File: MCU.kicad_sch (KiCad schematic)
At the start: 10 parts

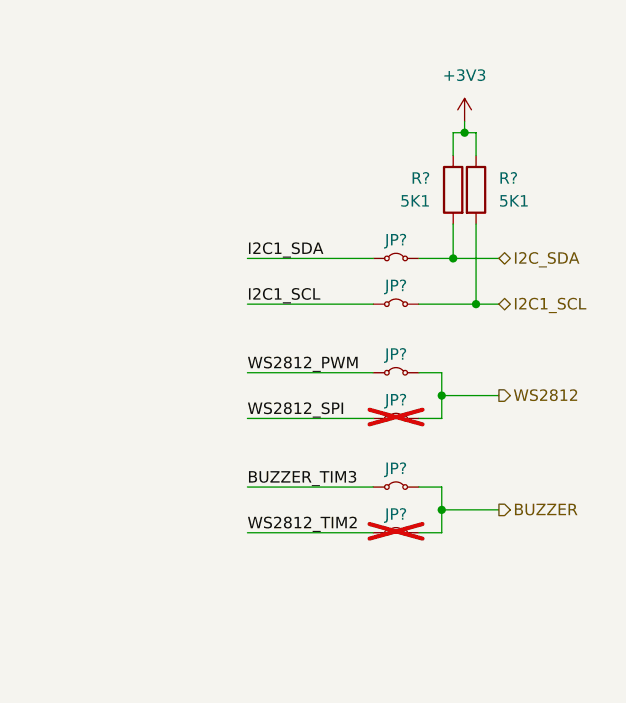
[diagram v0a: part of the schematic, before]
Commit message: Small changes
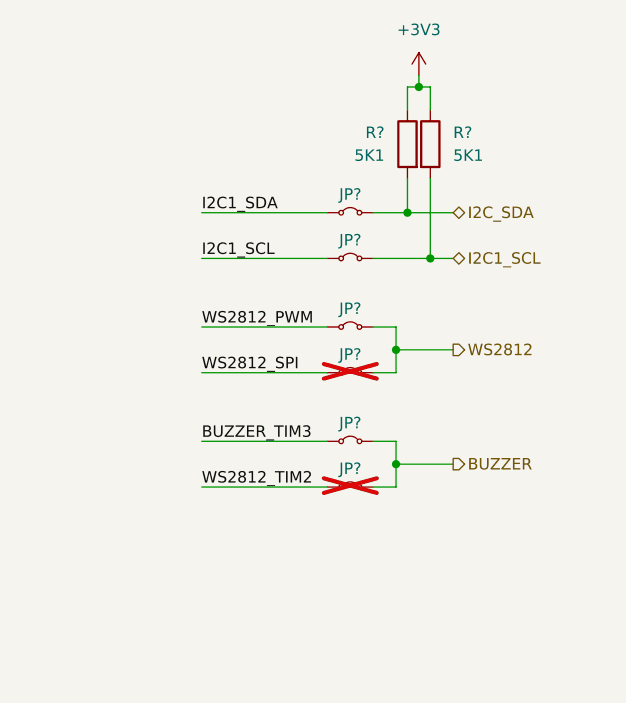
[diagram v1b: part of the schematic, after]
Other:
- moved on the sheet: JP?, R?
